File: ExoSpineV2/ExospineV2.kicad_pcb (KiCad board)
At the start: 2 copper layers, 80.4 x 72.4 mm, 51 parts, among them J1 GPIO, J11 JST PH 3pin, J12 2.54mm 4pin, J13 JST PH 5pin, J2 Screw Terminal 2pin 5mm, J21 JST PH 2pin, J22 JST PH 2pin, J23 JST PH 2pin, J3 Mounting Hole 2.7mm, J31 JST PH 3pin, J32 JST PH 3pin, J33 JST PH 3pin, J34 JST PH 3pin, J35 JST PH 3pin, J36 JST PH 3pin, J4 Mounting Hole 2.7mm, J5 Mounting Hole 2.7mm, J51 JST PH 2pin, J6 Mounting Hole 2.7mm, J61 JST PH 2pin, J71 JST PH 4pin, J72 JST PH 3pin, J73 JST PH 4pin, J74 JST PH 3pin, J75 JST PH 4pin, J76 JST PH 3pin, J77 JST PH 4pin, J78 JST PH 3pin, J81 JST PH 3pin, J82 JST PH 3pin, U1 MCP3008-I/SL, U2 74HC00D,653, U3 74HC00D,653

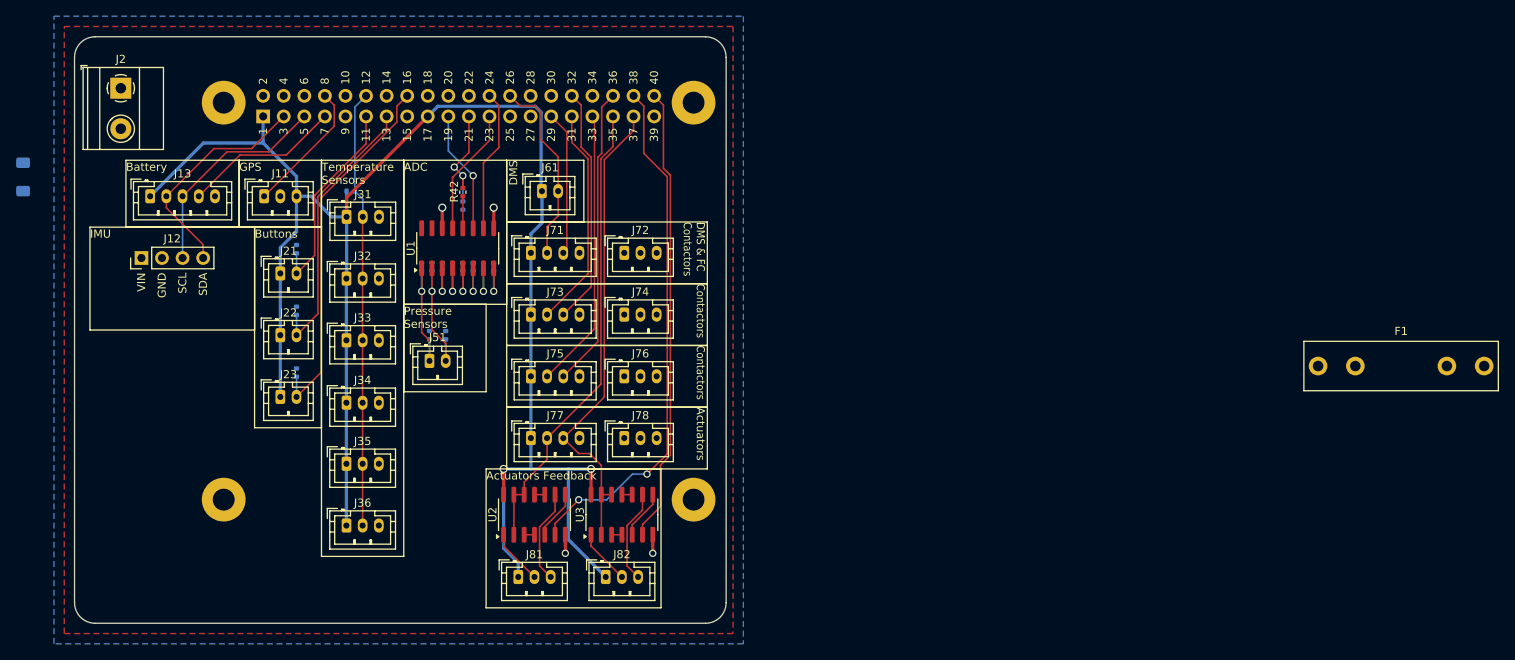
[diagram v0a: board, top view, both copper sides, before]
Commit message: clarified net names among other things
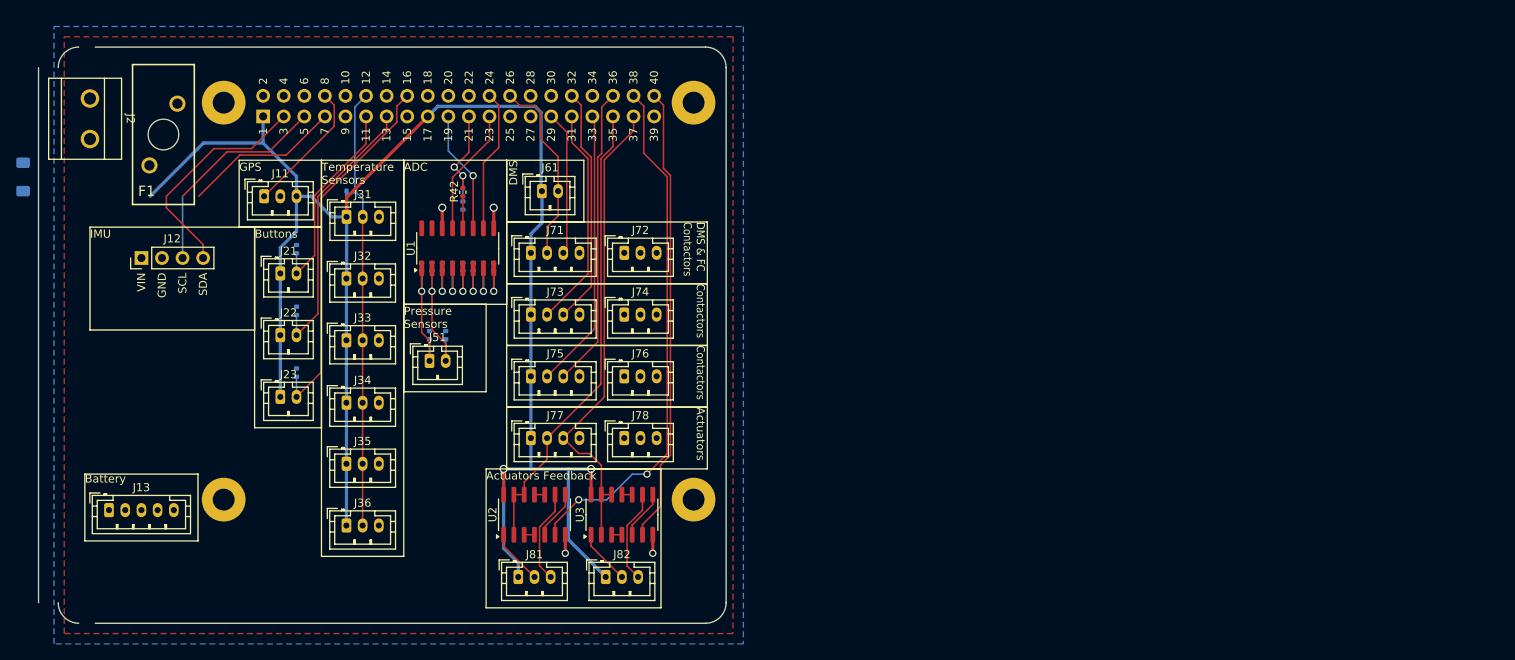
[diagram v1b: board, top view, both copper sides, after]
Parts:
- F1: value Fuse -> Fuse Holder; footprint Fuse:Fuseholder_Littelfuse_100_series_5x20mm -> ExoSpineV2:[Mouser]01530008(Littelfuse)
- J2: footprint TerminalBlock_Phoenix:TerminalBlock_Phoenix_MKDS-1,5-2_1x02_P5.00mm_Horizontal -> ExoSpineV2:[Exocet]XY126V-5.0-2P
- moved F1 145.4 mm to (96.1, 31.1), turned to 180 degrees
- moved J13 39.1 mm to (89.3, 77.5)
- moved J2 5.36 mm to (87.0, 29.2)
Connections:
- net /GPIO10/SPI0.MOSI renamed /ADC.MOSI
- net /GPIO11/SPI0.SCLK renamed /ADC.SCLK
- net /GPIO12/PWM0 renamed /Contactor4
- net /GPIO13/PWM1 renamed /Contactor5
- net /GPIO14/TXD0 renamed /GPS.TX
- net /GPIO16 renamed /Contactor6
- net /GPIO17 renamed /Button1
- net /GPIO18/PCM.CLK renamed /TemperatureSensors
- net /GPIO19/PCM.FS renamed /Actuator1
- net /GPIO20/PCM.DIN renamed /Actuator1.Feedback
- net /GPIO21/PCM.DOUT renamed /Actuator2.Feedback
- net /GPIO23 renamed /Button3
- net /GPIO26 renamed /Actuator2
- net /GPIO27 renamed /Button2
- net /GPIO2/SDA1 renamed /SDA
- net /GPIO3/SCL1 renamed /SCL
- net /GPIO4/GPCLK0 renamed /Battery.NALCC
- net /GPIO5 renamed /Contactor2
- net /GPIO6 renamed /Contactor3
- net /GPIO7/SPI0.CE1 renamed /Contactor1.DMS
- net /GPIO8/SPI0.CE0 renamed /ADC.Enable
- net /GPIO9/SPI0.MISO renamed /ADC.MISO
- J1 pad 10: /GPIO15/RXD0 -> unconnected-(J1-GPIO15/UART.RXD-Pad10)
- J1 pad 15: /GPIO22 -> unconnected-(J1-GPIO22-Pad15)
- J1 pad 18: /GPIO24 -> unconnected-(J1-GPIO24-Pad18)
- J1 pad 22: /GPIO25 -> unconnected-(J1-GPIO25-Pad22)
- J1 pad 27: /ID_SDA -> unconnected-(J1-ID.SD-Pad27)
- J1 pad 28: /ID_SCL -> unconnected-(J1-ID.SC-Pad28)
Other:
- board size 80.4 x 72.4 mm -> 84.9 x 71.1 mm
